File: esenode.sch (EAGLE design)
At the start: 11 parts, among them Q1 CSTCR6M00G53Z, U1 LPC11U6XJBD48, U2 RFM95W-868S2

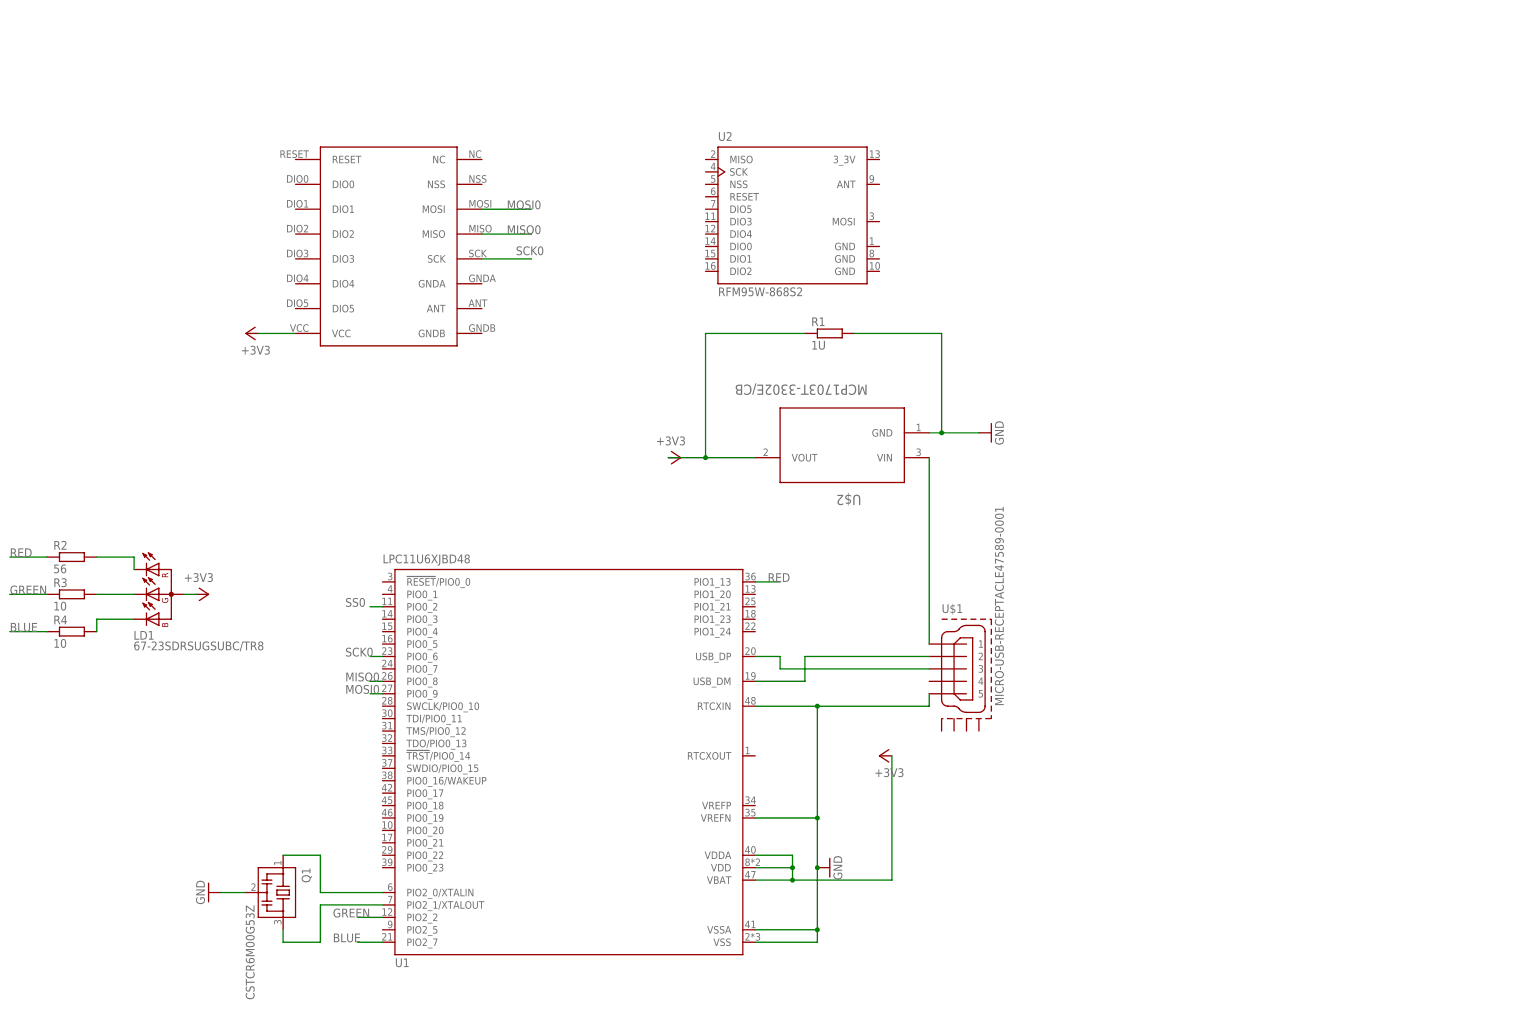
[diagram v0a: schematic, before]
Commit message: #challenge, then connect gpio to top bar and see if still possible lol
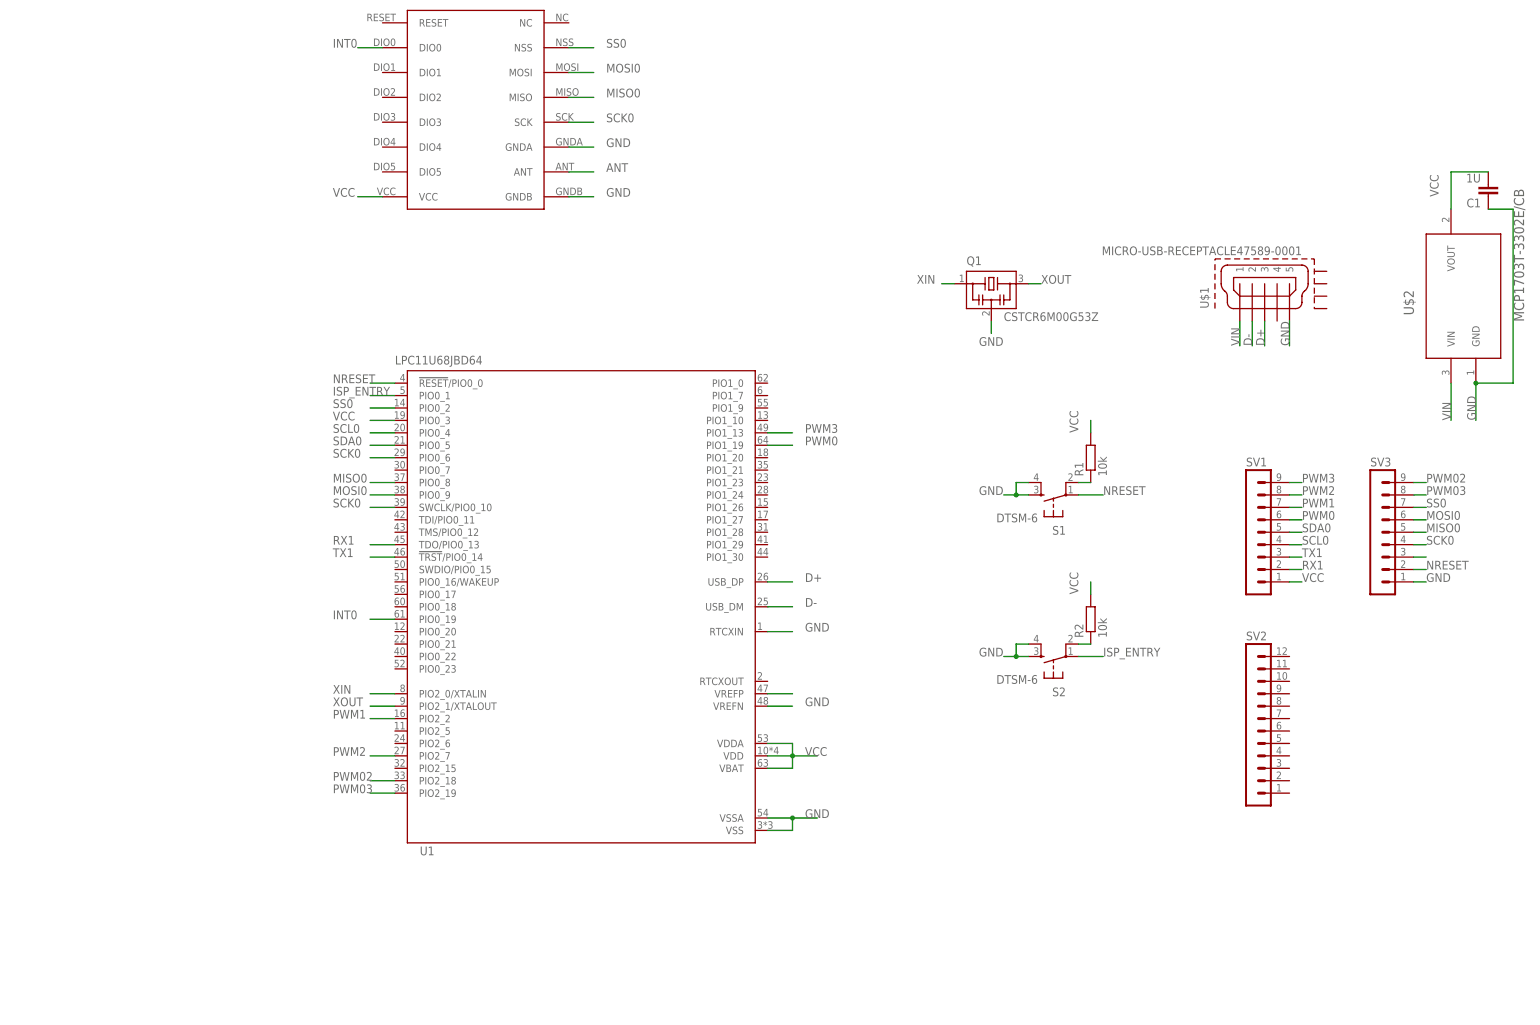
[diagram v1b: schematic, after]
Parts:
- removed LD1: 67-23SDRSUGSUBC/TR8, everlight:67-23SDRSUGSUBC/TR8
- removed R3, R4: 10, eagle-ltspice:RR0603
- removed U2: RFM95W-868S2, RFM95W-868S2:RFM95W-868S2
- added C1: 1U, rcl:C-EUC0805
- added S1, S2: DTSM-6, switch-tact:DTSM-6
- added SV1, SV3: (no value), con-lstb:MA09-1
- added SV2: (no value), con-lstb:MA12-1
- R1: value 1U -> 10k; device resistor:R-EU_R0603 -> rcl:R-EU_M0805
- R2: value 56 -> 10k; device eagle-ltspice:RR0603 -> rcl:R-EU_M0805
- U1: value LPC11U6XJBD48 -> LPC11U68JBD64; device NXP_60_26022015:LPC11U6XJBD48 -> NXP_60_26022015:LPC11U68JBD64
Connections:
- net N$1 renamed XIN
- net N$2 renamed XOUT
- net N$3 renamed D-
- net N$4 renamed D+
- net N$5 renamed VIN
- removed net +3V3: LD1.CA, R1.1, U$2.VOUT, U$3.VCC, U1.VBAT, U1.VDD, U1.VDDA
- removed net BLUE: R4.1, U1.PIO2_7
- removed net GREEN: R3.1, U1.PIO2_2
- removed net N$8: LD1.BC, R4.2
- removed net RED: R2.1, U1.PIO1_13
- new net ANT: U$3.ANT
- new net INT0: U$3.DIO0, U1.PIO0_19
- new net ISP_ENTRY: S2.1, U1.PIO0_1
- new net N$18: SV3.3
- new net N$4: U1.VREFP
- new net NRESET: S1.1, SV3.2, U1.!RESET!/PIO0_0
- new net PWM0: SV1.6, U1.PIO1_19
- new net PWM02: SV3.9, U1.PIO2_18
- new net PWM03: SV3.8, U1.PIO2_19
- new net PWM1: SV1.7, U1.PIO2_2
- new net PWM2: SV1.8, U1.PIO2_7
- new net PWM3: SV1.9, U1.PIO1_13
- new net RX1: SV1.2, U1.TDO/PIO0_13
- new net SCL0: SV1.4, U1.PIO0_4
- new net SDA0: SV1.5, U1.PIO0_5
- new net TX1: SV1.3, U1.!TRST!/PIO0_14
- new net VCC: C1.2, R1.2, R2.2, SV1.1, U$2.VOUT, U$3.VCC, U1.PIO0_3, U1.VBAT, U1.VDD, U1.VDDA
- net GND: now also C1.1, S1.3, S1.4, S2.3, S2.4, SV3.1, U$3.GNDA, U$3.GNDB; no longer R1.2
- net MISO0: now also SV3.5
- net MOSI0: now also SV3.6
- net N$6: now also R2.1, S2.2; no longer LD1.RC, R2.2
- net N$7: now also R1.1, S1.2; no longer LD1.GC, R3.2
- net SCK0: now also SV3.4, U1.SWCLK/PIO0_10
- net SS0: now also SV3.7, U$3.NSS
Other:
- moved on the sheet: Q1, R1, R2, U$1, U$2
